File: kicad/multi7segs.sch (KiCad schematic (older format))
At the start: 12 parts

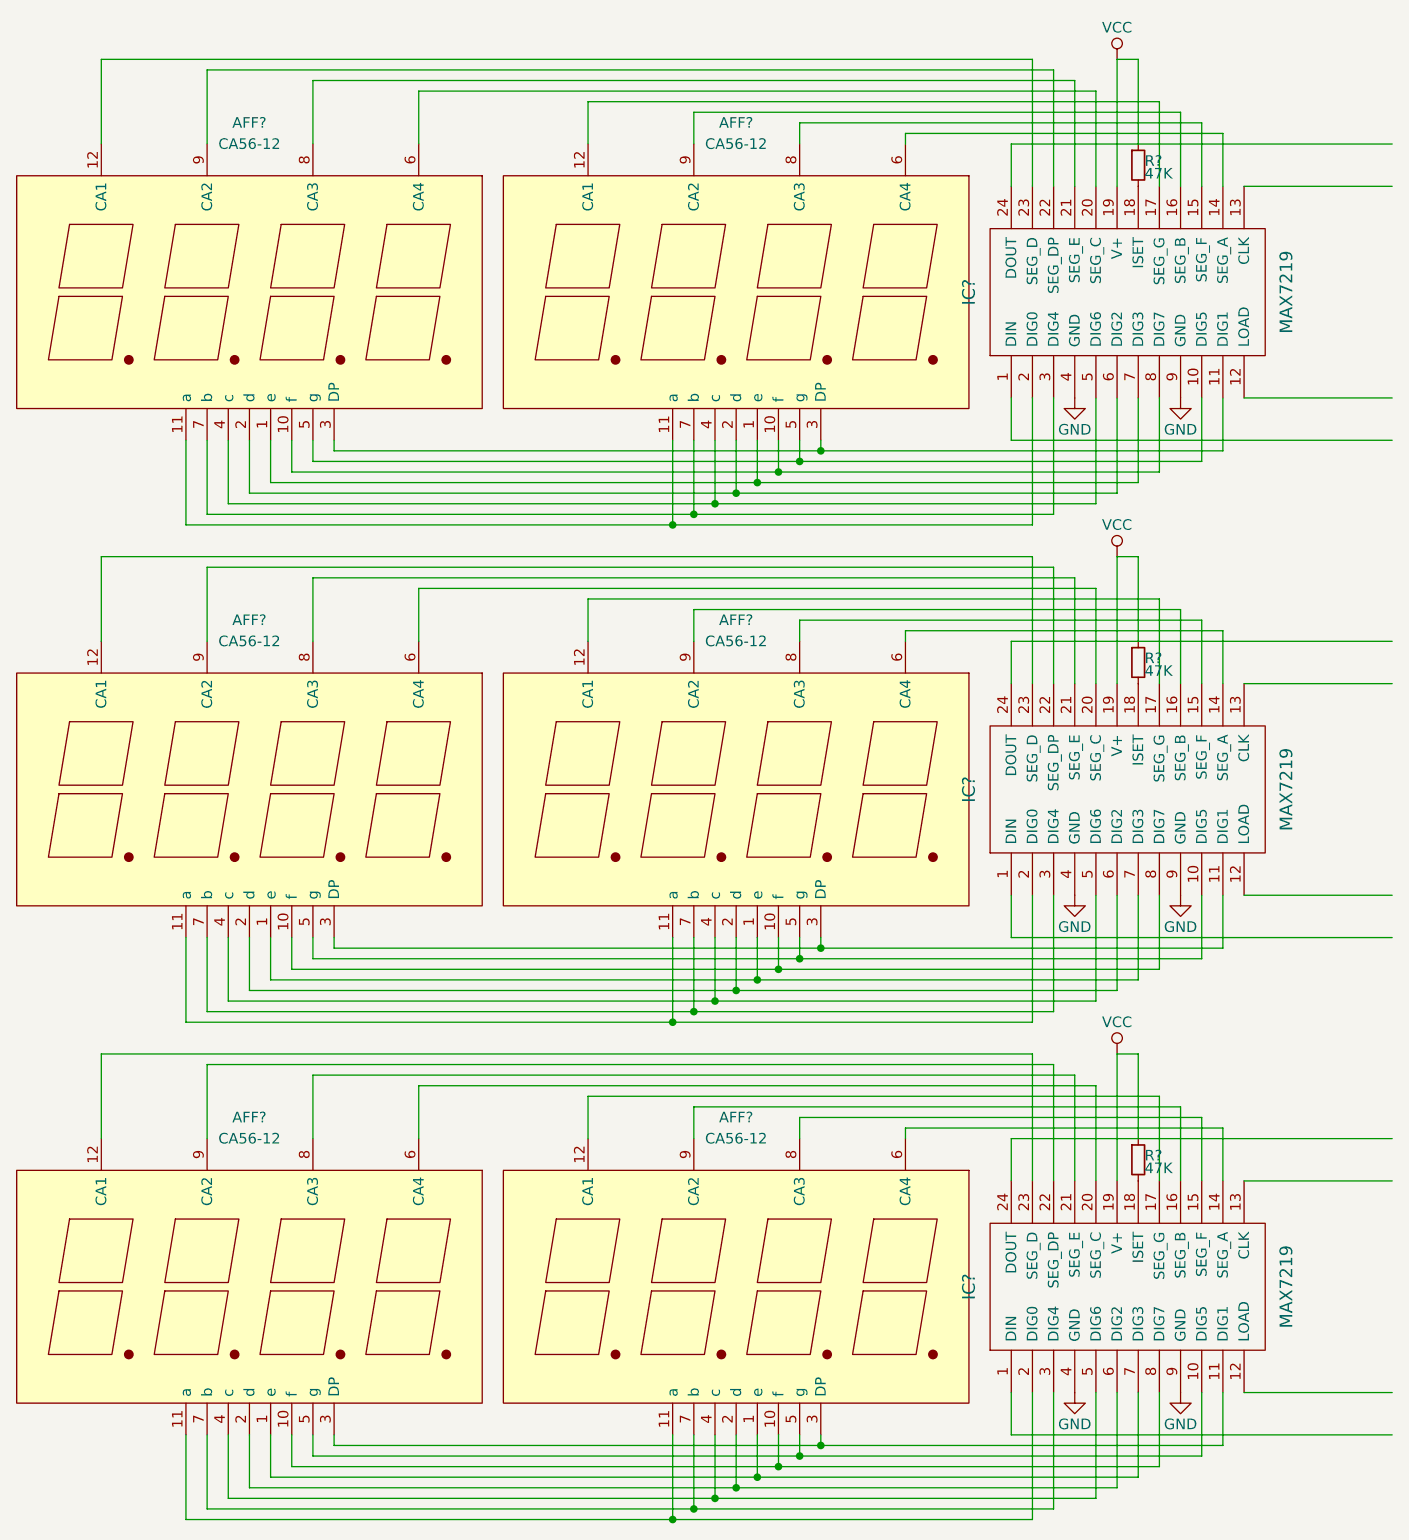
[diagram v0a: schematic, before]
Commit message: "Realistic" wiring
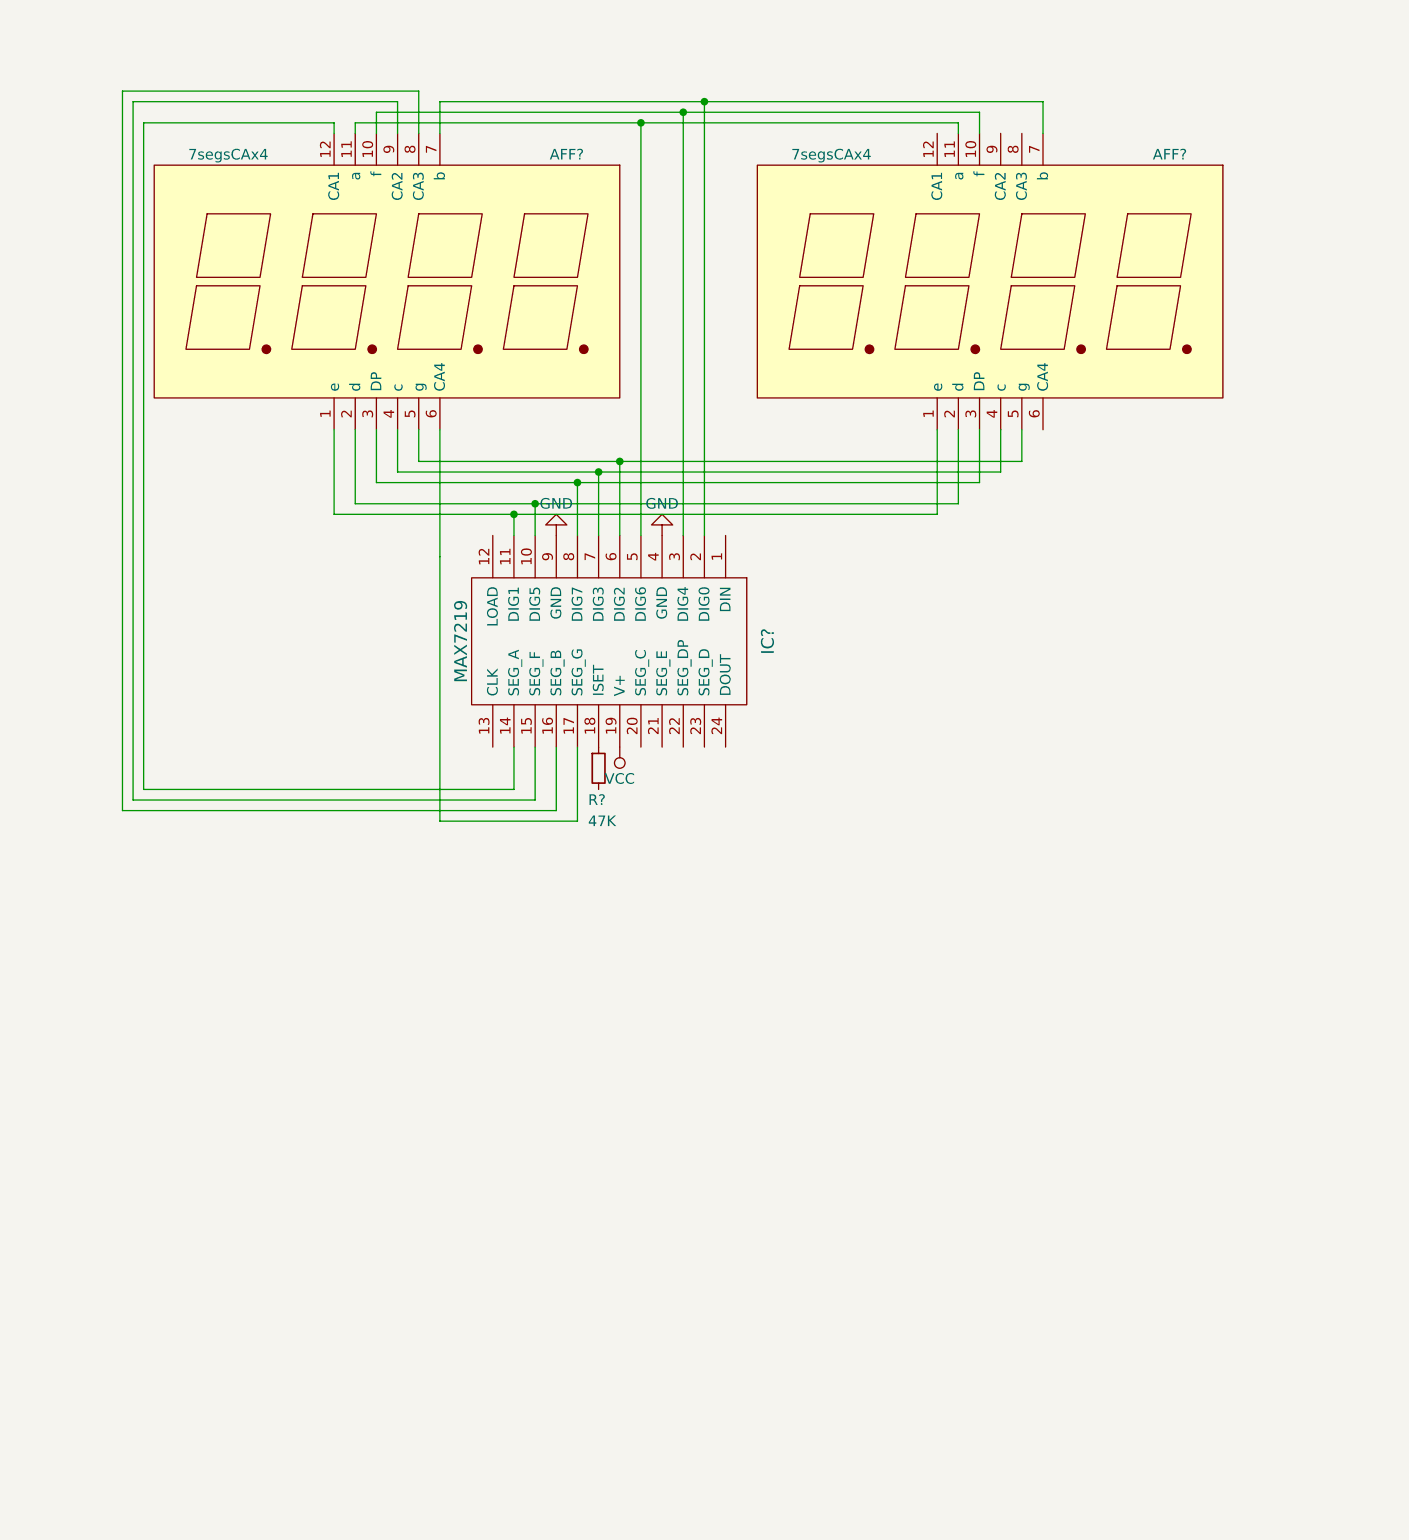
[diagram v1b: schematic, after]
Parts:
- removed AFF? (x6): CA56-12, symbol CA56-12
- removed IC? (x2): MAX7219, symbol MAX7219
- removed R? (x2): 47K, symbol R_Small
- added AFF? (x2): 7segsCAx4, symbol 7segsCAx4
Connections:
- wire segments 219 -> 60
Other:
- moved on the sheet: IC?, R?
